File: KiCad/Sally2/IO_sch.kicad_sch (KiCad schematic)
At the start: 42 parts, among them J12 Drive 1-4, J13 OPT, J14 Special_Func, J15 TX GND RX, J16 + RI -, J17 RS232, J18 IN RDY CMD OUT GND, J19 Centronics, J20 Conn_01x13, J8 Conn_01x13, U10 MAX232, U11 74LS06, U12 74LS06, U13 Z84C30, U14 74LS244, U15 74LS273, U16 74LS244, U8 74LS273, U9 WD1772_PHY

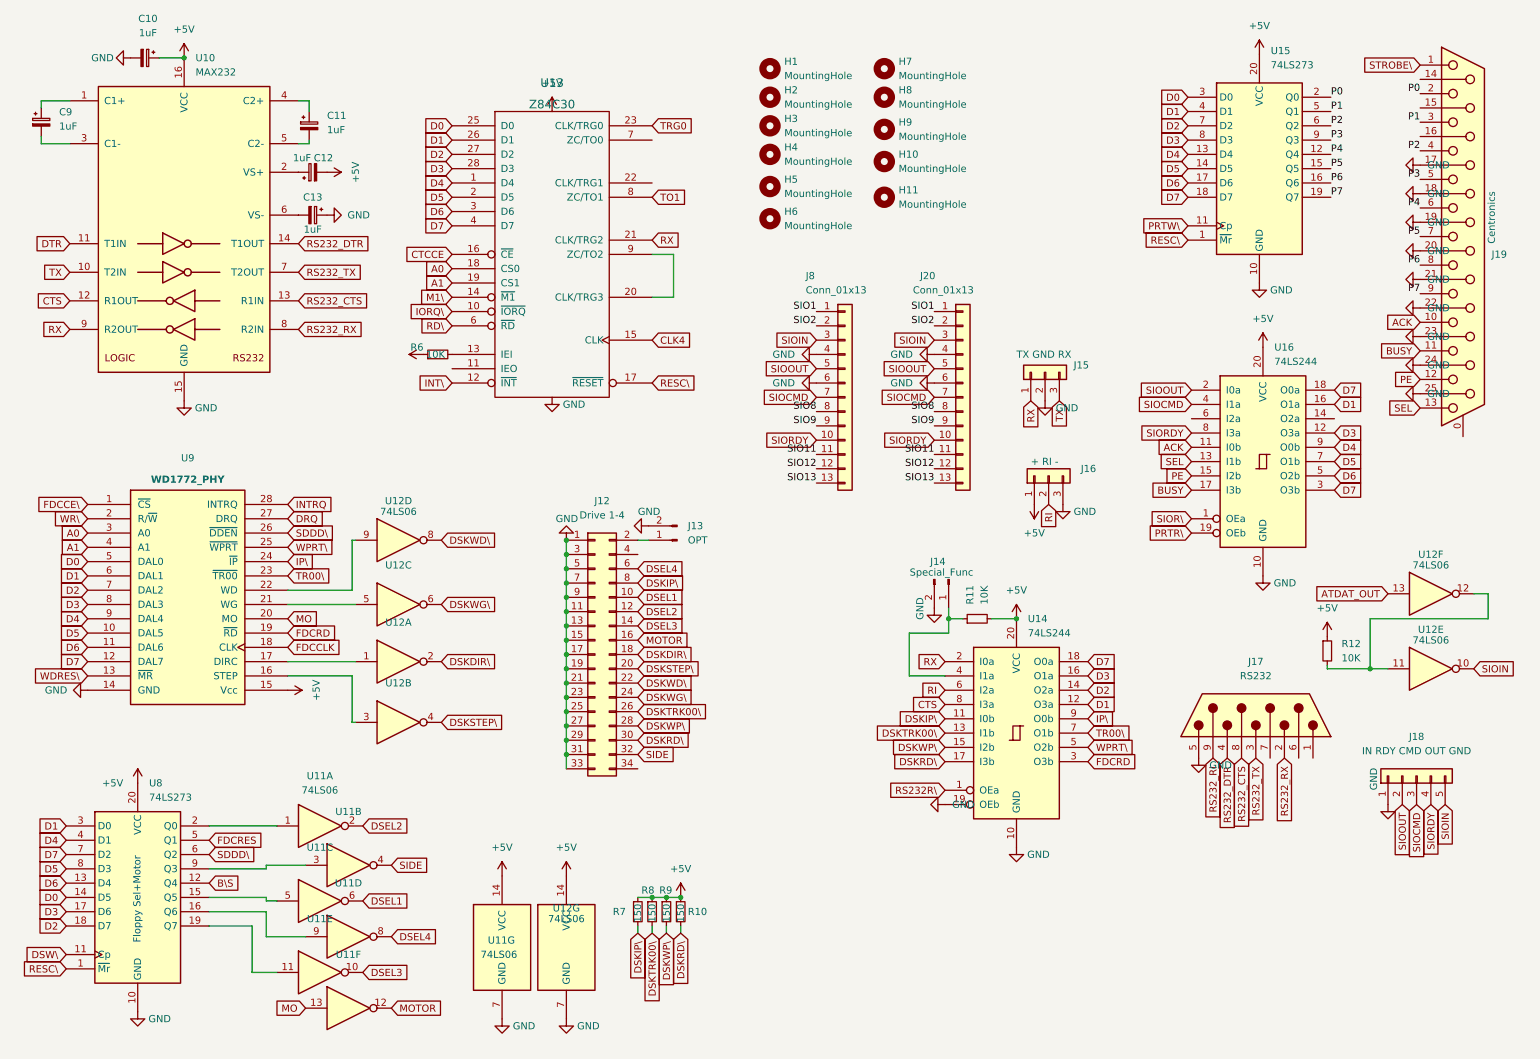
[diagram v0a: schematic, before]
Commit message: KiCad merges from Marc
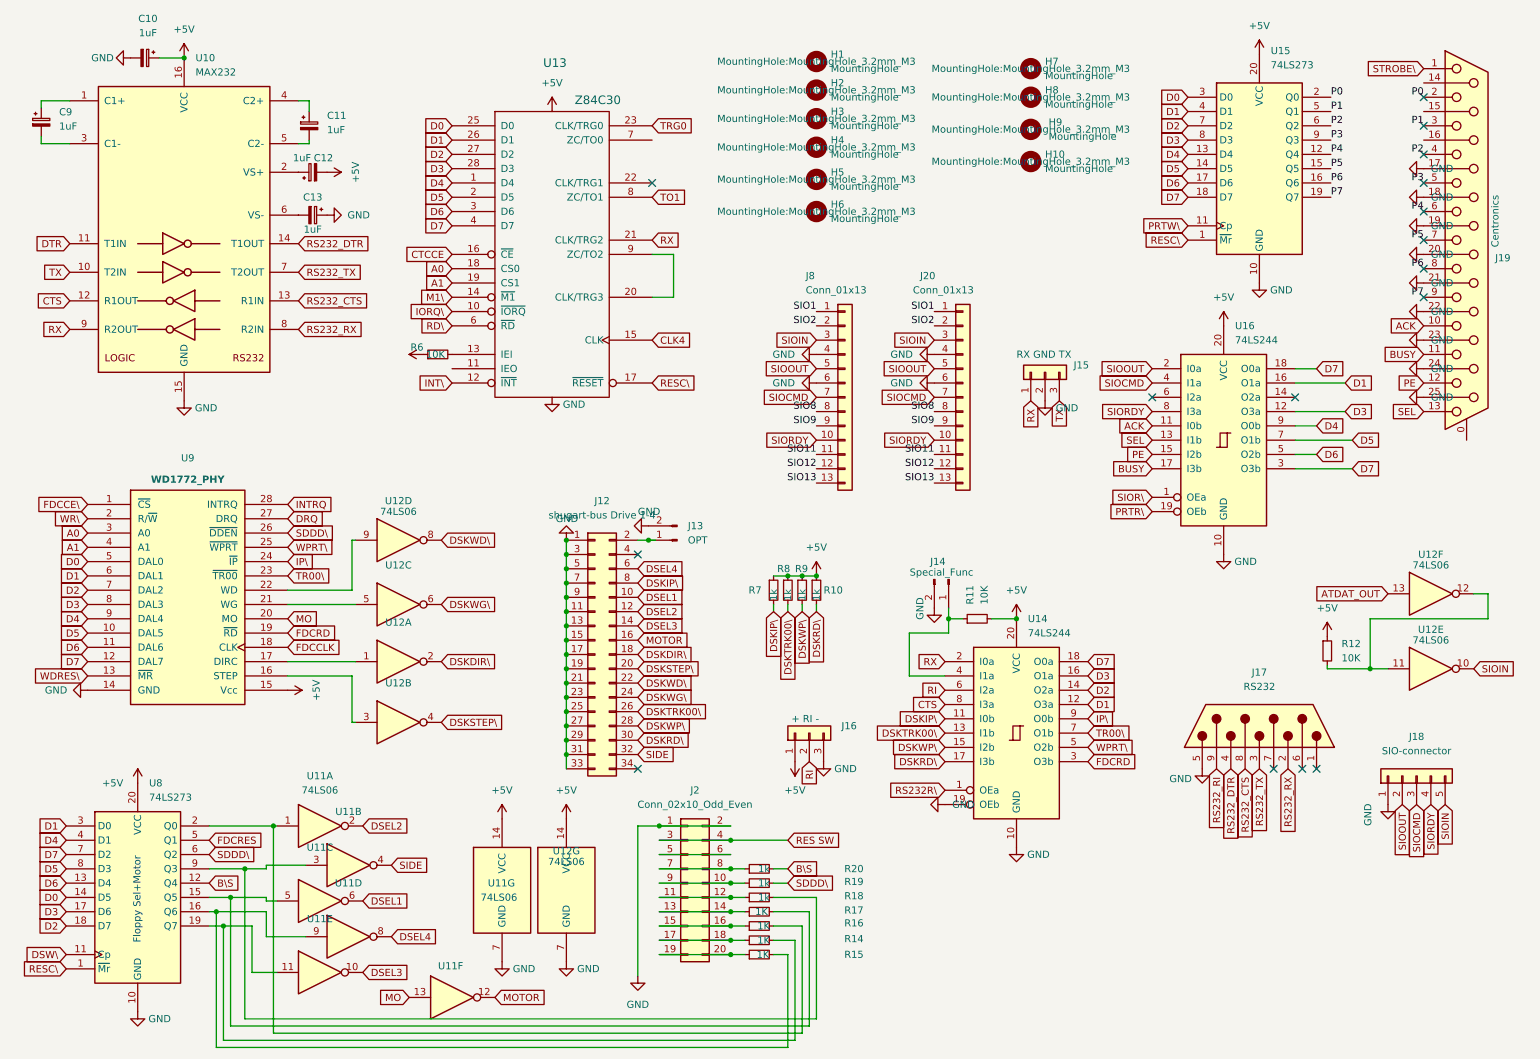
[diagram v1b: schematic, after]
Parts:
- removed H11: MountingHole, MountingHole:MountingHole_4.3mm_M4, symbol Mechanical:MountingHole
- added J2: Conn_02x10_Odd_Even, Connector_PinHeader_2.54mm:PinHeader_2x10_P2.54mm_Horizontal, symbol Connector_Generic:Conn_02x10_Odd_Even
- added R14, R15, R16, R17: 1K, Resistor_THT:R_Axial_DIN0207_L6.3mm_D2.5mm_P10.16mm_Horizontal, symbol Device:R_Small
- added R18, R19, R20: 1k, Resistor_THT:R_Axial_DIN0207_L6.3mm_D2.5mm_P10.16mm_Horizontal, symbol Device:R_Small
- H1, H10, H2, H3, H4, H5, H6, H7, H8, H9: footprint MountingHole:MountingHole_4.3mm_M4 -> MountingHole:MountingHole_3.2mm_M3
- J12: value Drive 1-4 -> shugart-bus Drive 1-4
- J15: value TX GND RX -> RX GND TX
- J16: value + RI - -> + RI -
- J17: footprint Connector_Dsub:DSUB-9_Male_Horizontal_P2.77x2.84mm_EdgePinOffset4.94mm_Housed_MountingHolesOffset7.48mm -> Connector_Dsub:DSUB-9_Male_Horizontal_P2.77x2.84mm_EdgePinOffset9.90mm_Housed_MountingHolesOffset11.32mm
- J18: value IN RDY CMD OUT GND -> SIO-connector
- R10, R7, R8, R9: value 150 -> 1k
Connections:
- net B\S: now also R20.2
- net GND: now also J2.1 (Pin_1), J2.2 (Pin_2)
- net SDDD\: now also R19.2
- net at U11.5, U8.15 (Q5): now also R17.2
- net at U11.9, U8.16 (Q6): now also R15.2
- net at U11.11, U8.19 (Q7): now also R14.2
- net at U11.1, U8.2 (Q0): now also R16.2
- net at U11.3, U8.9 (Q3): now also R18.2
- new net: J2.10 (Pin_10), J2.9 (Pin_9), R19.1
- new net: J2.11 (Pin_11), J2.12 (Pin_12), R18.1
- new net: J2.13 (Pin_13), J2.14 (Pin_14), R17.1
- new net: J2.15 (Pin_15), J2.16 (Pin_16), R16.1
- new net: J2.17 (Pin_17), J2.18 (Pin_18), R14.1
- new net: J2.19 (Pin_19), J2.20 (Pin_20), R15.1
- new net: J2.5 (Pin_5), J2.6 (Pin_6)
- new net: J2.7 (Pin_7), J2.8 (Pin_8), R20.1
- new net RES SW: J2.3 (Pin_3), J2.4 (Pin_4)
- no-connect marks 0 -> 16
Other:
- moved on the sheet: H1, H10, H2, H3, H4, H5, H6, H7, H8, H9, J16, J17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
